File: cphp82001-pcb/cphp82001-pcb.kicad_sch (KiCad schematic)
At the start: 32 parts, among them J1 USB_B_Micro, J2 PAD+, J3 PAD-, Q1 2N7002, U1 BQ21040, U2 TLV75801, U3 MAX40203AUK, U4 TPS3808DBV, U6 NCP360SNT

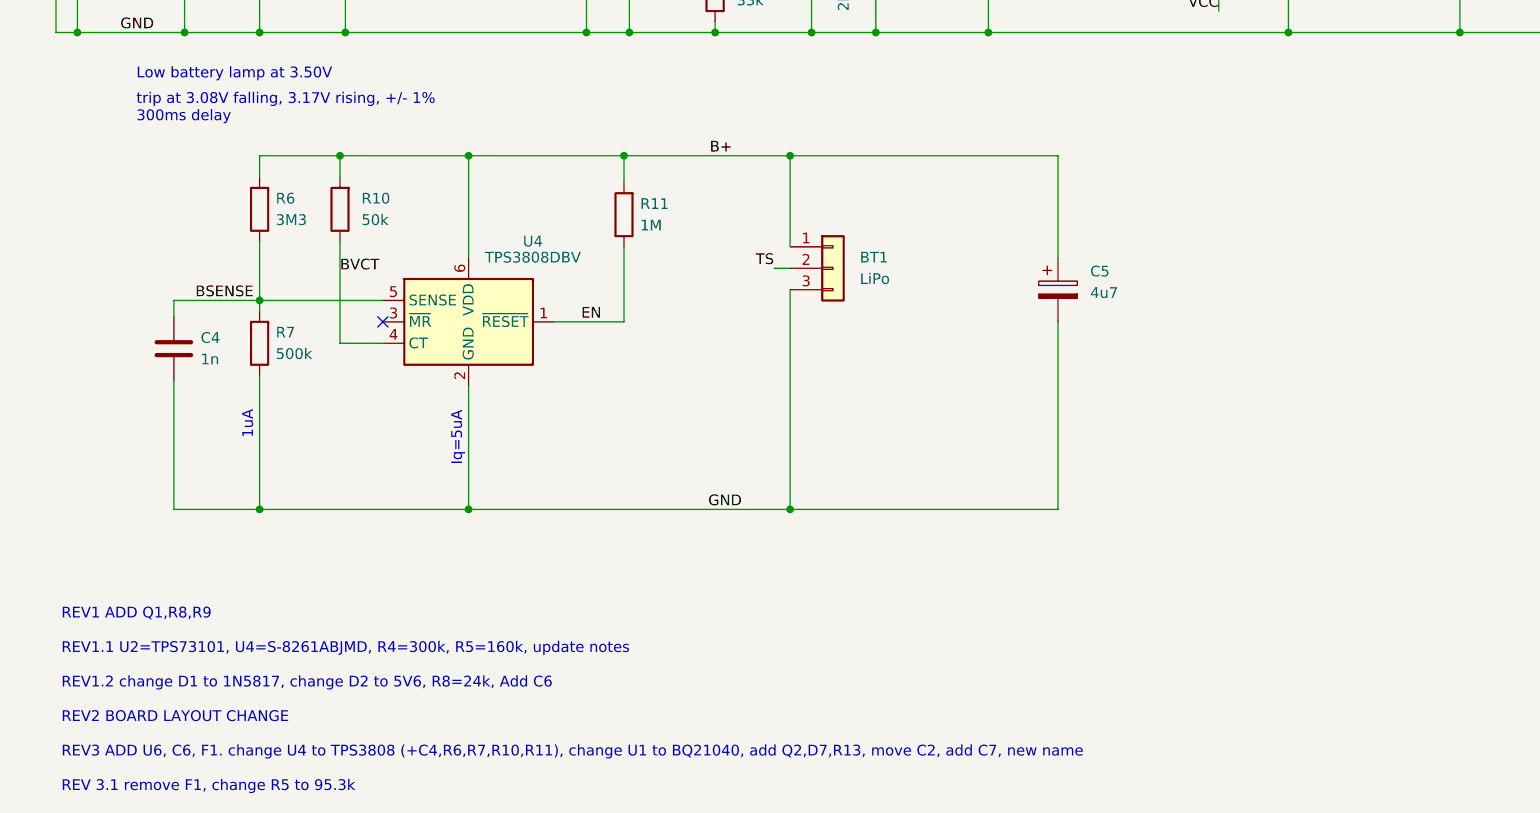
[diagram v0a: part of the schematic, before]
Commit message: Rev3.2
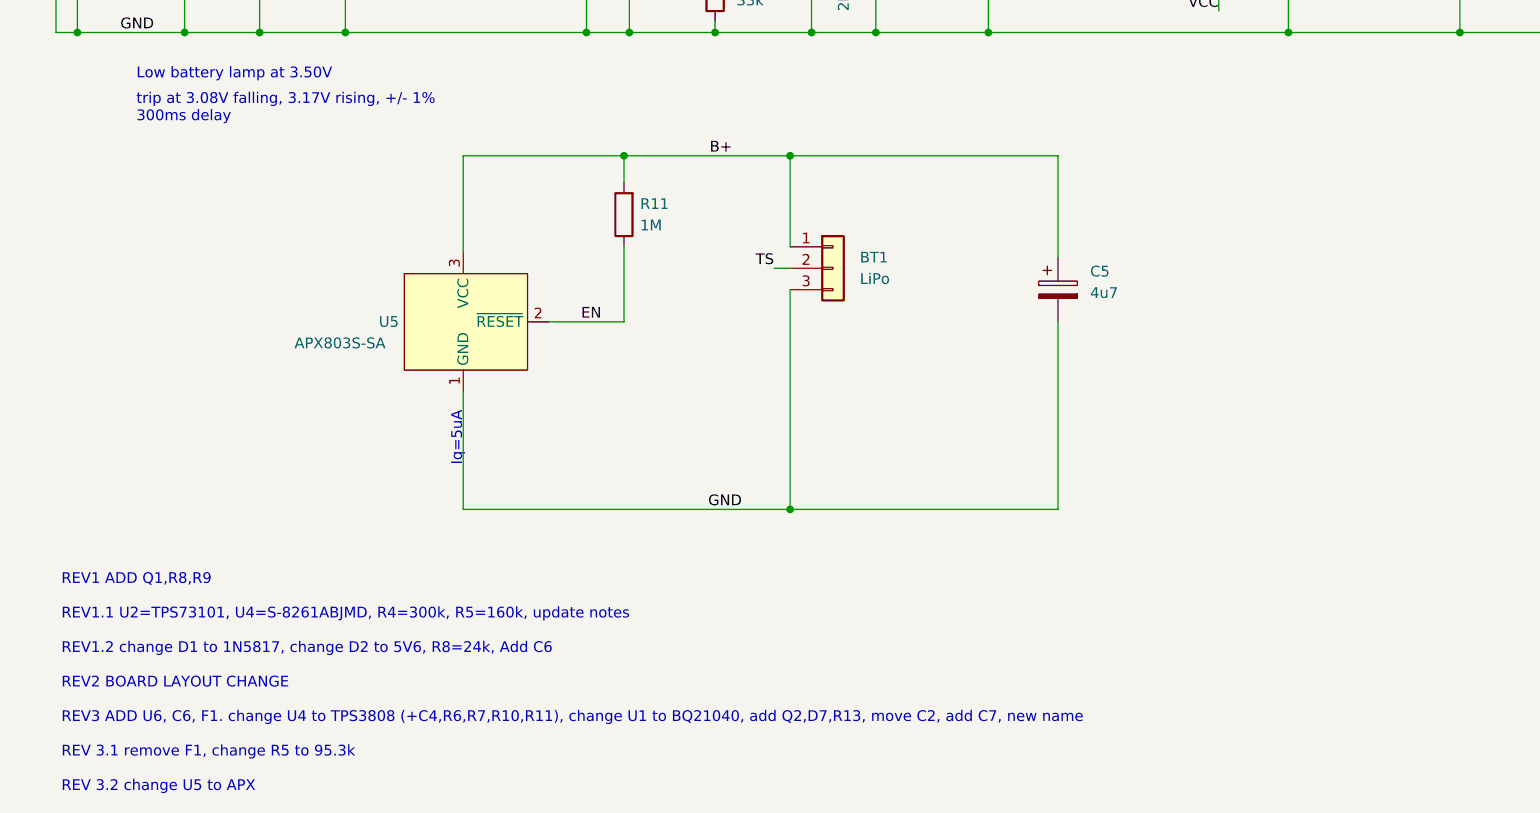
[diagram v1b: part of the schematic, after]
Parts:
- removed C4: 1n, Capacitor_SMD:C_0805_2012Metric, symbol Device:C
- removed R10: 50k, Resistor_SMD:R_0805_2012Metric, symbol Device:R
- removed R6: 3M3, Resistor_SMD:R_0805_2012Metric, symbol Device:R
- removed R7: 500k, Resistor_SMD:R_0805_2012Metric, symbol Device:R
- removed U4: TPS3808DBV, george:SOT-23-6_TI_DBV6, symbol Power_Supervisor:TPS3808DBV
- added U5: APX803S-SA, Package_TO_SOT_SMD:SOT-23-3, symbol kicad_george:APX803S-XXSA
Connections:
- net B+: now also U5.3 (VCC)
- net EN: now also U5.2 (~{RESET})
- net GND: now also U5.1 (GND)
- no-connect marks 5 -> 4
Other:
- note added: "REV1 ADD Q1,R8,R9 REV1.1 U2=TPS73101, U4=S-8261ABJMD, R4=300k, R5=160k, update notes REV1.2 change D1 to 1N5817, change D2 to 5V6, R8=24k, Add C6 REV2 BOARD LAYOUT CHANGE REV3 ADD U6, C6, F1. change U4 to TPS3808 (+C4,R6,R7,R10,R11), change U1 to BQ21040, add Q2,D7,R13, move C2, add C7, new name REV 3.1 remove F1, change R5 to 95.3k REV 3.2 change U5 to APX"
- note removed: "1uA"
- note removed: "REV1 ADD Q1,R8,R9 REV1.1 U2=TPS73101, U4=S-8261ABJMD, R4=300k, R5=160k, update notes REV1.2 change D1 to 1N5817, change D2 to 5V6, R8=24k, Add C6 REV2 BOARD LAYOUT CHANGE REV3 ADD U6, C6, F1. change U4 to TPS3808 (+C4,R6,R7,R10,R11), change U1 to BQ21040, add Q2,D7,R13, move C2, add C7, new name REV 3.1 remove F1, change R5 to 95.3k"

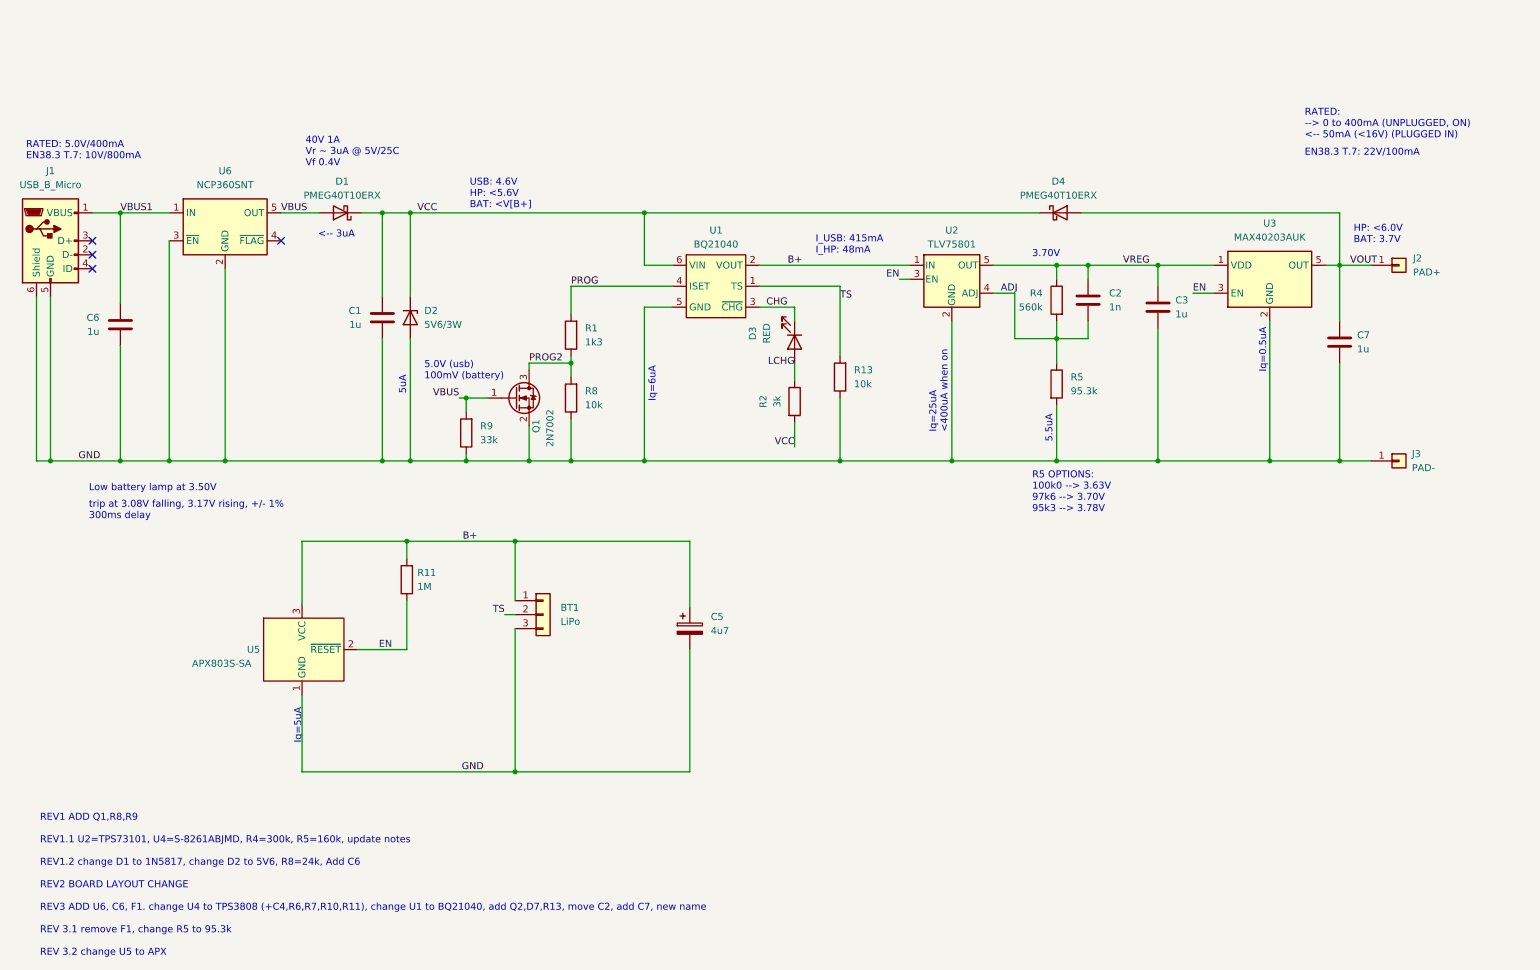
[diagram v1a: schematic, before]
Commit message: rev3.3
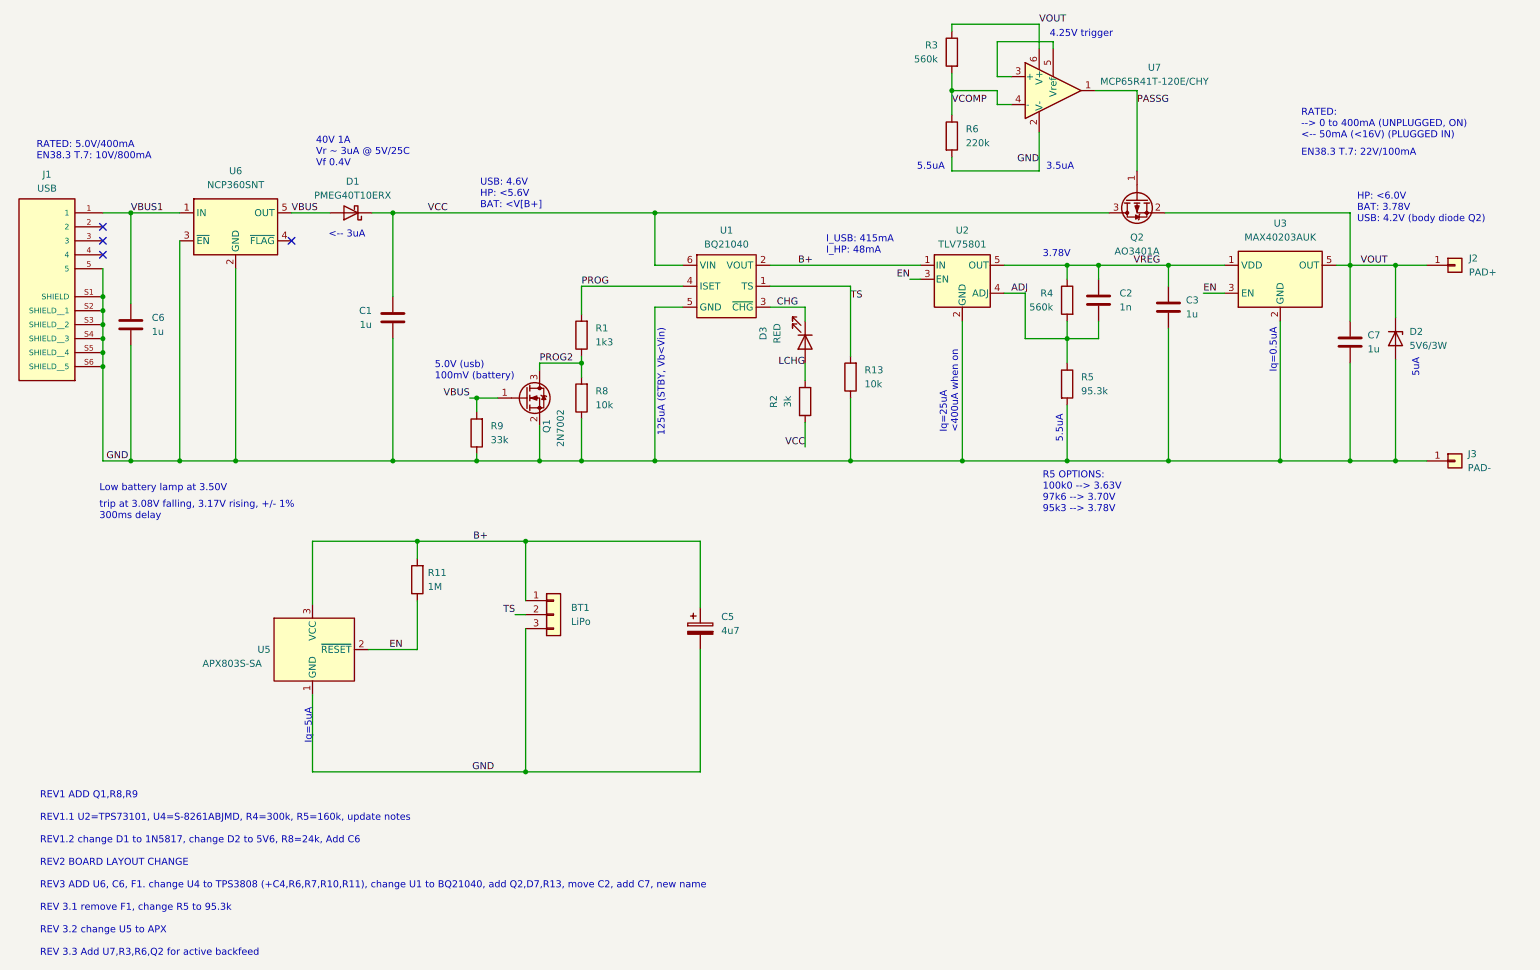
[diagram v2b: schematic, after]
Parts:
- removed D4: PMEG40T10ERX, Diode_SMD:D_SOD-123, symbol Diode:1N5819
- removed J1: USB_B_Micro, george:USB_ALIEX_4LEG, symbol Connector:USB_B_Micro
- added J1: USB, mod_local:AMPHENOL_10118194-0001LF, symbol amphenol_10118194:10118194-0001LF
- added Q2: AO3401A, Package_TO_SOT_SMD:SOT-23, symbol Transistor_FET:AO3401A
- added R3: 560k, Resistor_SMD:R_0805_2012Metric, symbol Device:R
- added R6: 220k, Resistor_SMD:R_0805_2012Metric, symbol Device:R
- added U7: MCP65R41T-120E/CHY, george:SOT-23-6_TI_DBV6, symbol Comparator:MCP65R41
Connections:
- net GND: now also J1.5, J1.S1 (SHIELD), J1.S2 (SHIELD__1), J1.S3 (SHIELD__2), J1.S4 (SHIELD__3), J1.S5 (SHIELD__4), J1.S6 (SHIELD__5), R6.2, U7.2 (V-)
- net VBUS1: now also J1.1
- net VCC: now also Q2.3 (D); no longer D2.1 (K)
- net VOUT: now also D2.1 (K), Q2.2 (S), R3.1, U7.6 (V+)
- new net: U7.3 (+), U7.5 (Vref)
- new net PASSG: Q2.1 (G), U7.1
- new net VCOMP: R3.2, R6.1, U7.4 (-)
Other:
- note added: "125uA (STBY, Vb<Vin)"
- note added: "3.5uA"
- note added: "3.78V"
- note added: "4.25V trigger"
- note added: "HP: <6.0V BAT: 3.78V USB: 4.2V (body diode Q2)"
- note added: "REV1 ADD Q1,R8,R9 REV1.1 U2=TPS73101, U4=S-8261ABJMD, R4=300k, R5=160k, update notes REV1.2 change D1 to 1N5817, change D2 to 5V6, R8=24k, Add C6 REV2 BOARD LAYOUT CHANGE REV3 ADD U6, C6, F1. change U4 to TPS3808 (+C4,R6,R7,R10,R11), change U1 to BQ21040, add Q2,D7,R13, move C2, add C7, new name REV 3.1 remove F1, change R5 to 95.3k REV 3.2 change U5 to APX REV 3.3 Add U7,R3,R6,Q2 for active back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"
- note removed: "3.70V"
- note removed: "HP: <6.0V BAT: 3.7V"
- note removed: "Iq=6uA"
- note removed: "REV1 ADD Q1,R8,R9 REV1.1 U2=TPS73101, U4=S-8261ABJMD, R4=300k, R5=160k, update notes REV1.2 change D1 to 1N5817, change D2 to 5V6, R8=24k, Add C6 REV2 BOARD LAYOUT CHANGE REV3 ADD U6, C6, F1. change U4 to TPS3808 (+C4,R6,R7,R10,R11), change U1 to BQ21040, add Q2,D7,R13, move C2, add C7, new name REV 3.1 remove F1, change R5 to 95.3k REV 3.2 change U5 to APX"
- moved on the sheet: BT1, C1, C2, C3, C5, C6, C7, D1, D2, D3, J2, J3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
